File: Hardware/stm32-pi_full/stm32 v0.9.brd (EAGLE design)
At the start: 131.4 x 105.8 mm, 273 parts, among them J1 SOLDERJUMPERNO, Q1 MMBT3906, Q2 MMBT3904, Q3 MMBT3904, U1 ESP32-WROOM-32D, Y1 6MM_3.5MM_CRYSTAL

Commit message: minor, uipdate BoMs
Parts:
- R21: value 0R -> 2k
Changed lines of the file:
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@@
 <attribute name="VALUE" x="11.495" y="57.635" size="1.27" layer="27" rot="R270"/>
 </element>
-<element name="R21" library="resistor" package="R0603" value="0R" x="76.883209375" y="56.964225" smashed="yes">
+<element name="R21" library="resistor" package="R0603" value="2k" x="76.883209375" y="56.964225" smashed="yes">
 <attribute name="NAME" x="78.810725" y="59.036134375" size="1.27" layer="25" rot="R180"/>
 <attribute name="VALUE" x="76.248209375" y="55.059225" size="1.27" layer="27"/>

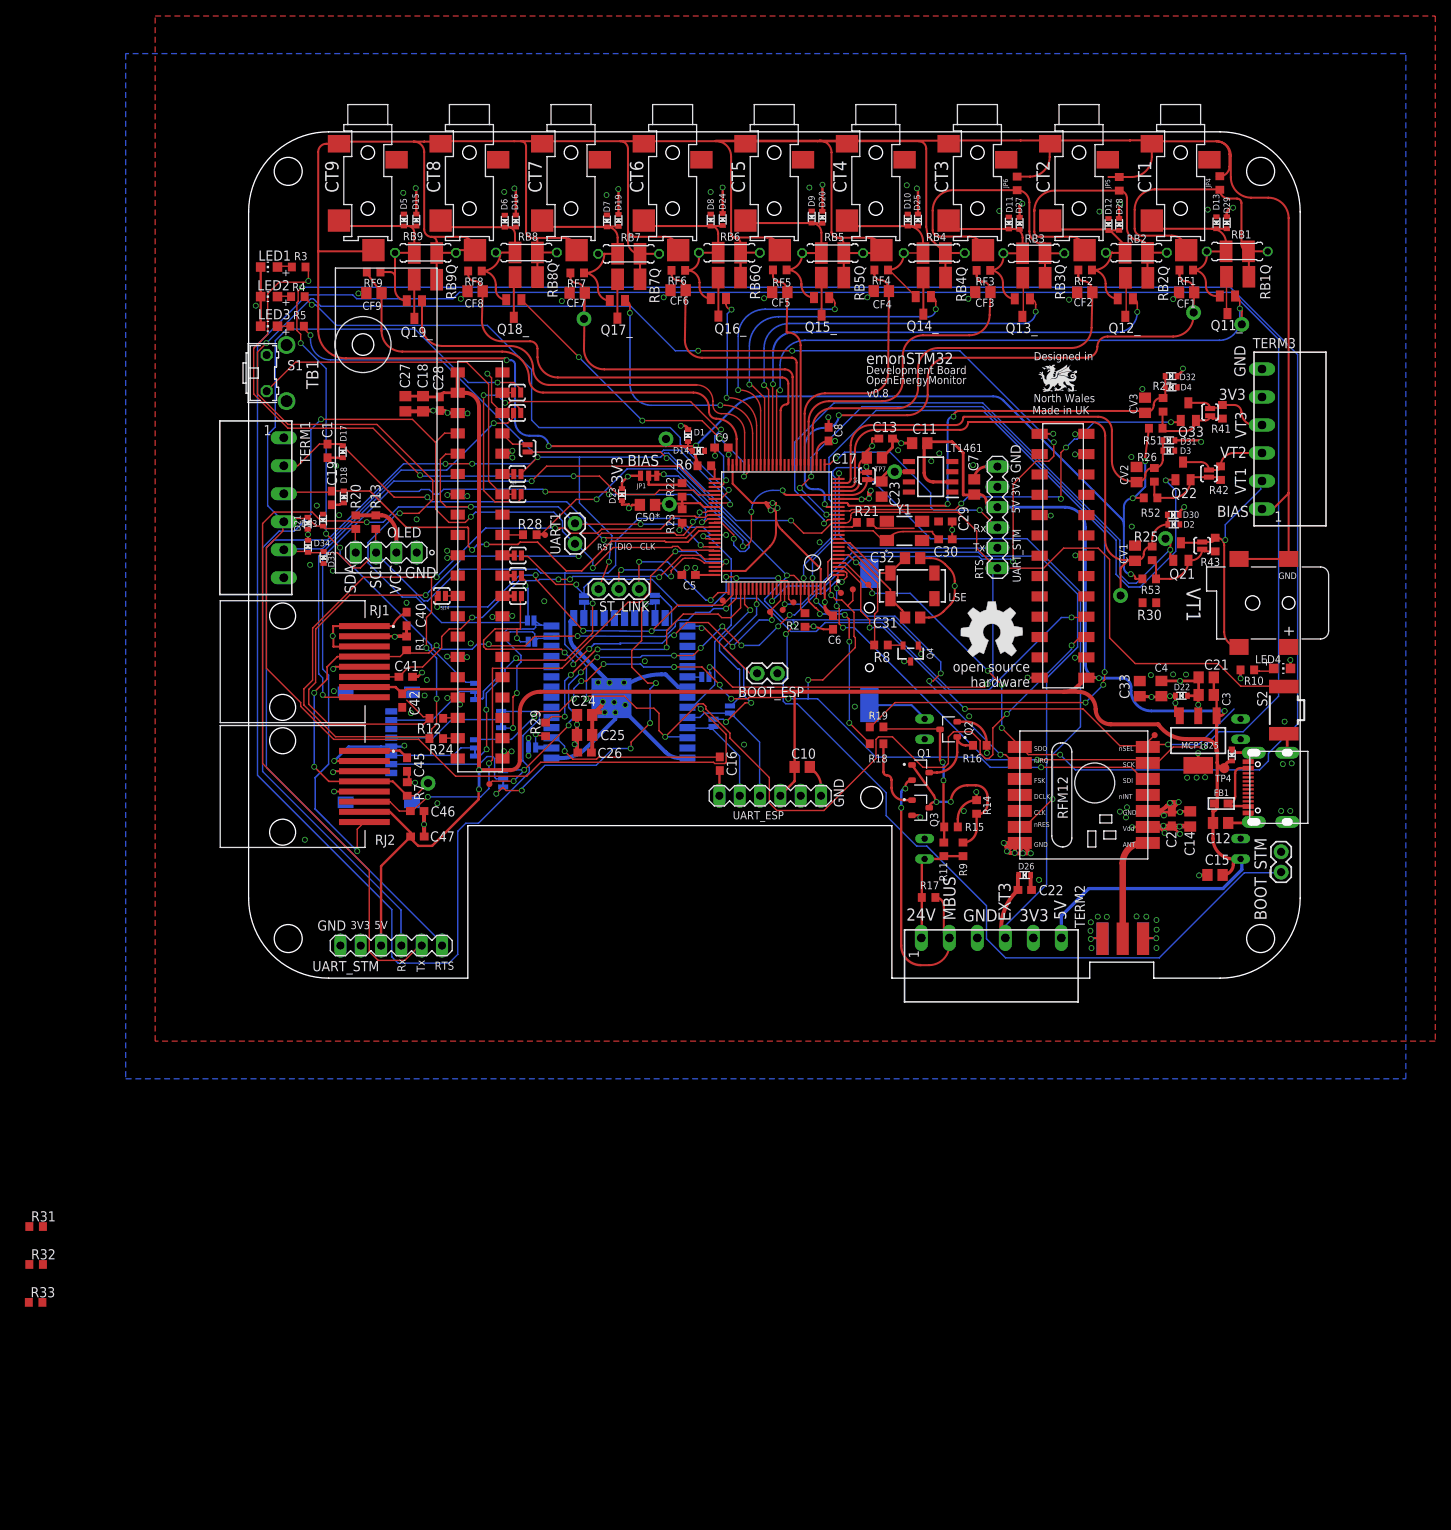
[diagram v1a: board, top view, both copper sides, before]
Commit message: minor changes, some checks on proto v0.8 done.
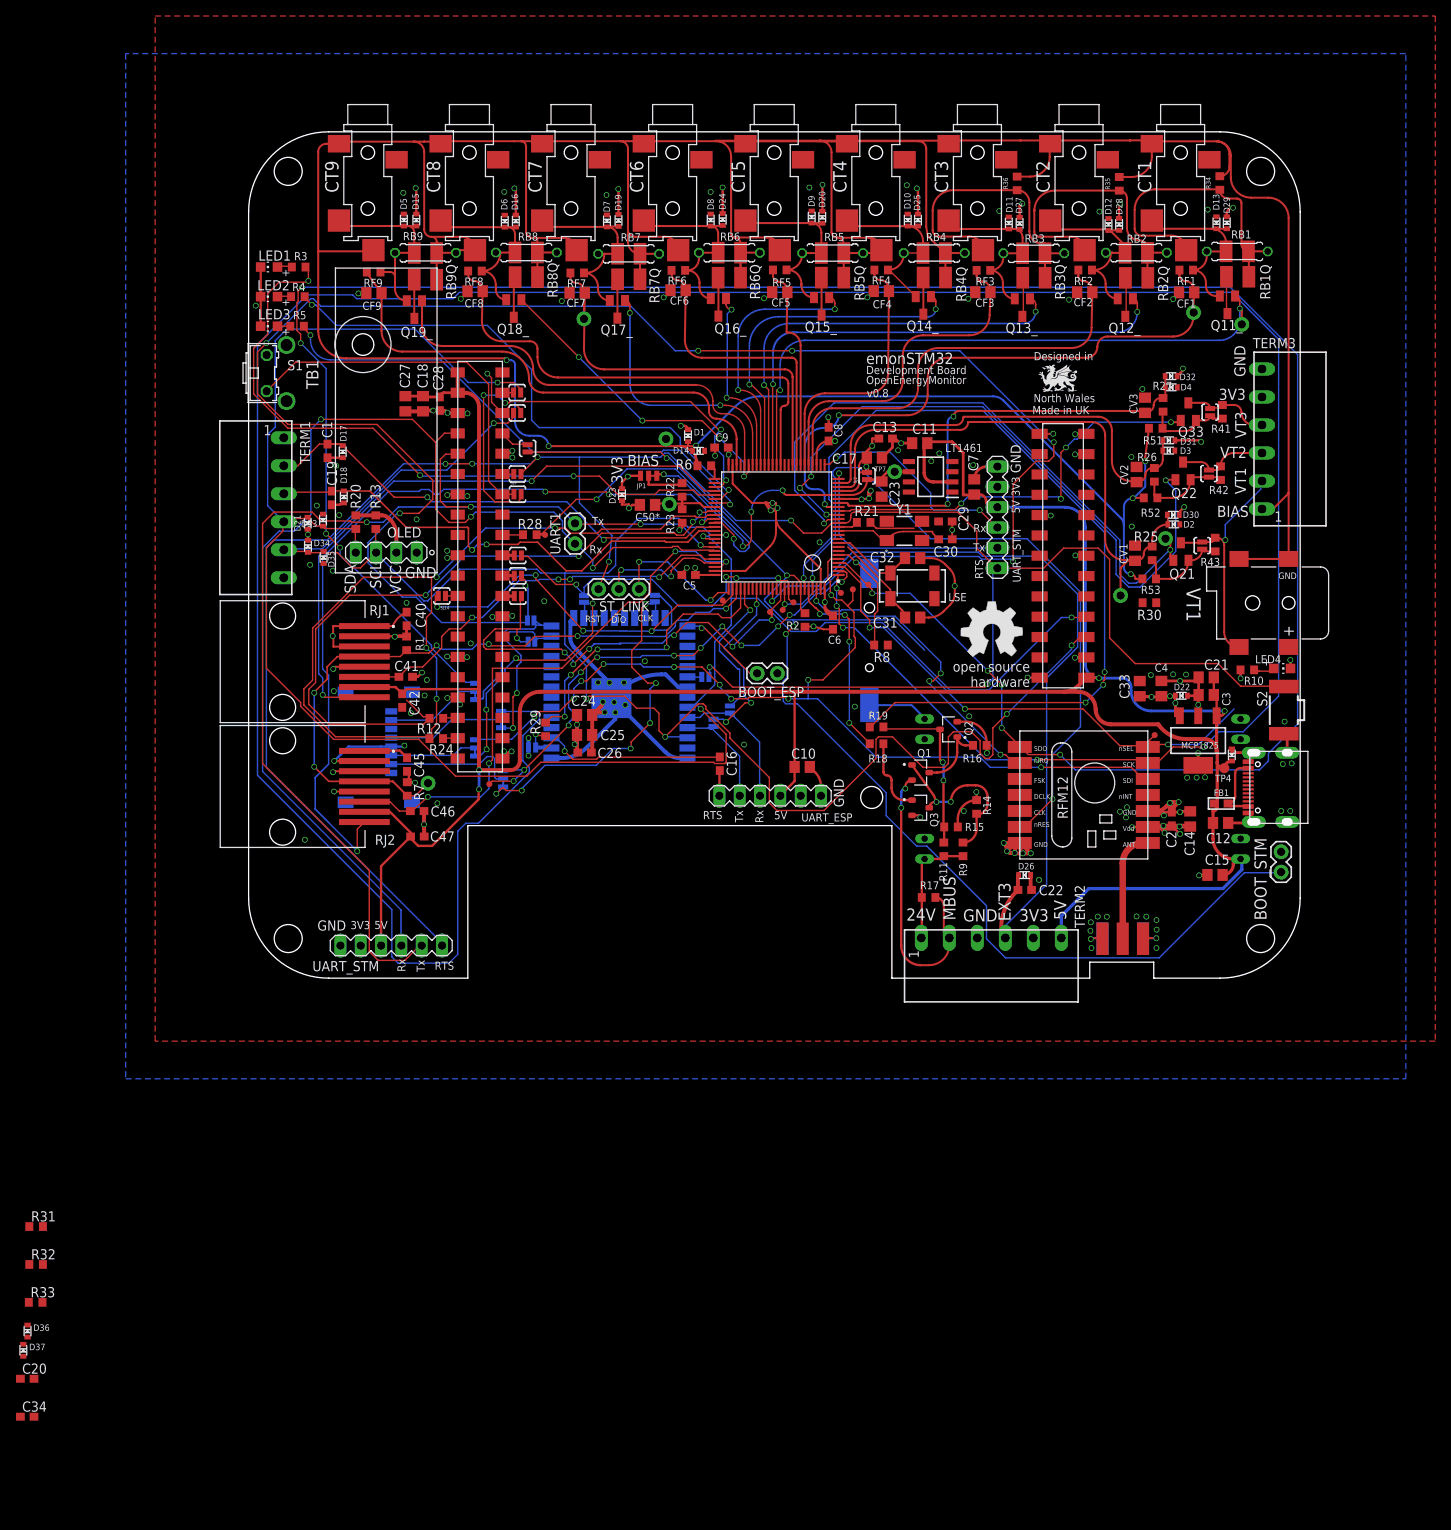
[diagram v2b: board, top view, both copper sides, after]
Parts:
- removed Q4: (no value), microbuilder:SOT23-R
- added C20, C34: 100nF, rcl:C0603
- added D36, D37: ESD5Z3.3T1G, microbuilder:SOD-523
- R34, R35, R36: value (none) -> 0R
- R8: value 1.5k -> 100k
- renumbered JP4 to R34, JP5 to R35, JP6 to R36
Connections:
- new net N$19: D37.K, R8.1
- net +3V3: no longer Q4.3
- net +5V: now also D36.A
- net GND: now also C20.2; no longer Q4.1
- net N$16: now also D36.K, D37.A; no longer Q4.2, R8.1
- net NRST_STM: now also C34.1, C34.2
- net VBAT: now also C20.1
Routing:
- net N$16: track 1.93 -> 0.00 mm
- net BIAS: track 588.4 -> 587.1 mm
- net GND: track 296.9 -> 295.6 mm, vias 143 -> 142
- net +3V3: track 143.8 -> 143.0 mm, vias 41 -> 40

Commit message: Various checks.
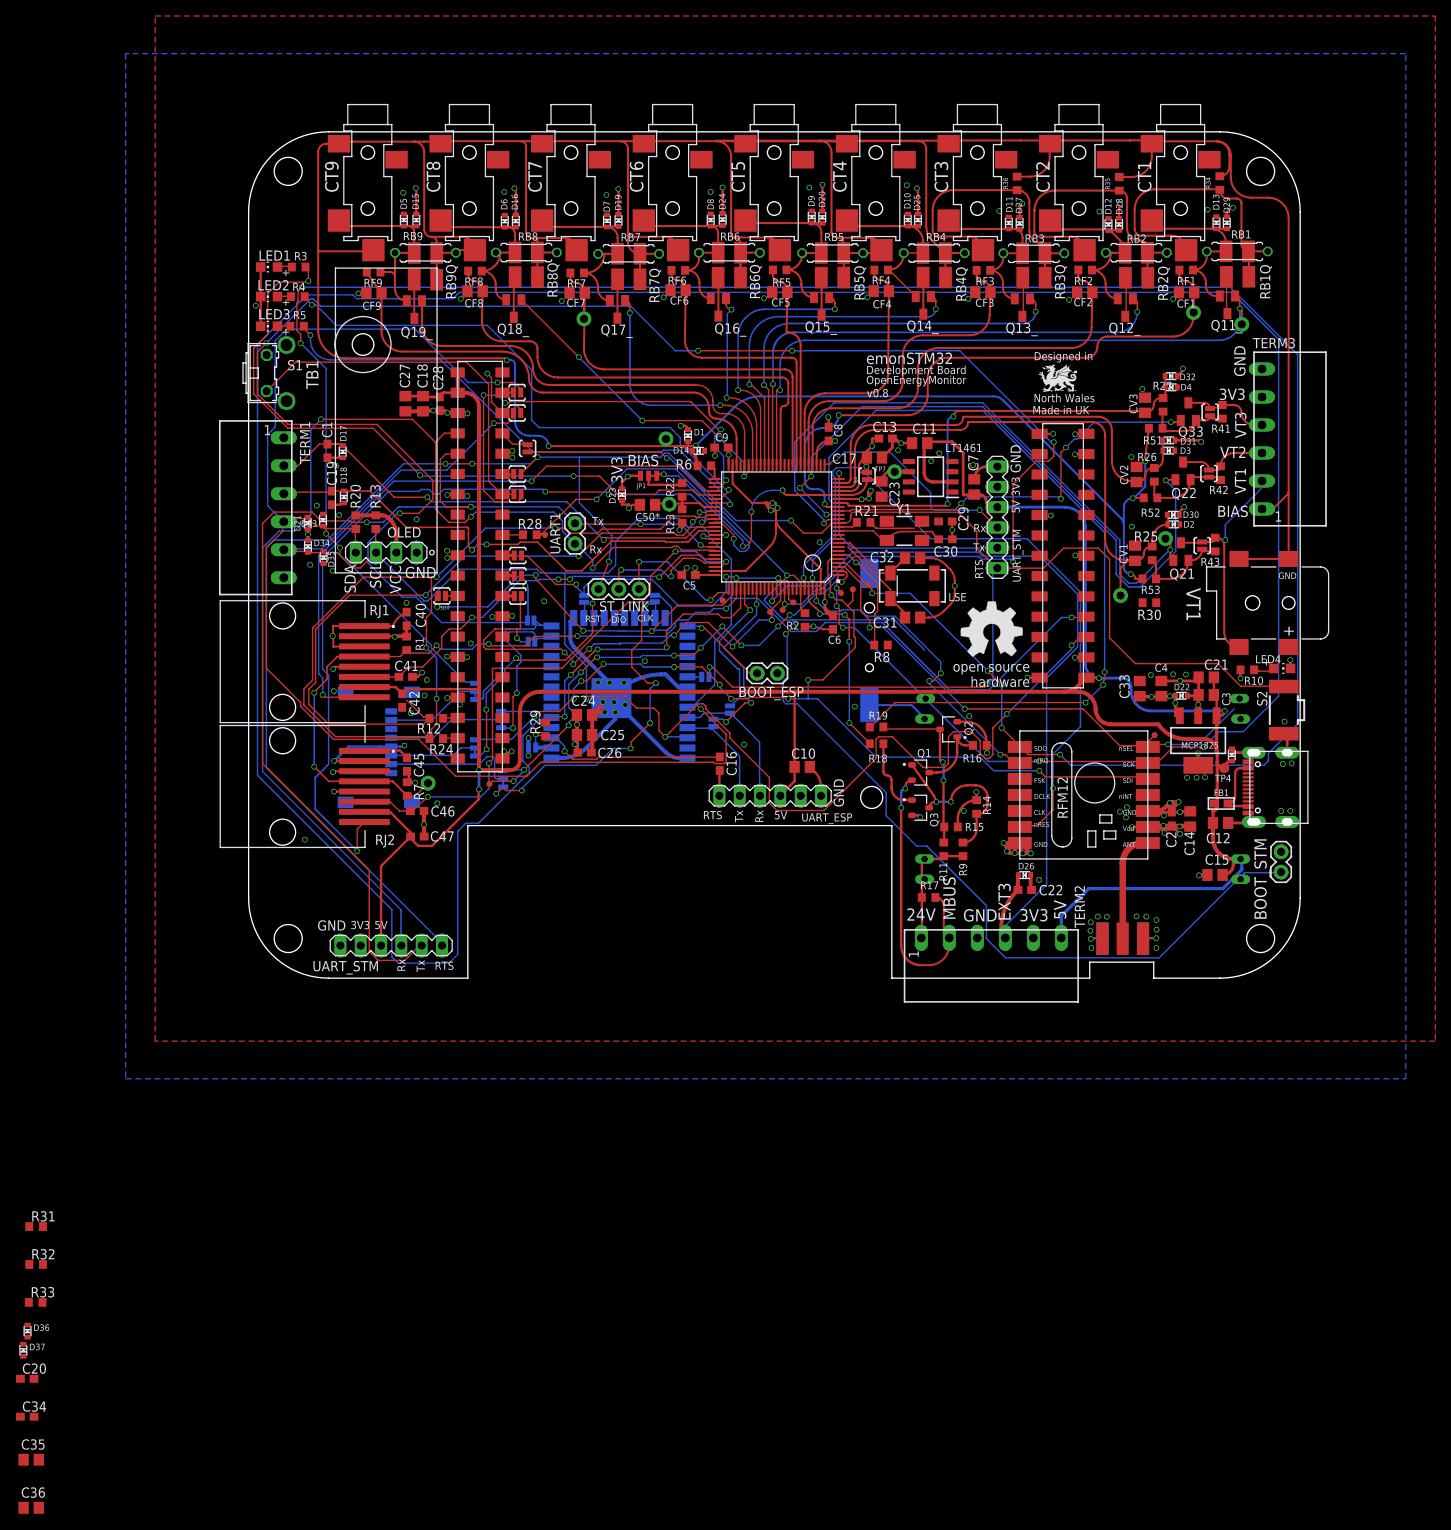
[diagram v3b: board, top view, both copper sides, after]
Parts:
- added C35, C36: 2.2uF, rcl:C0805
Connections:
- net BIAS: now also C35.1, C36.1
- net GND: now also C35.2, C36.2
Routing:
- net RST_RFM: track 86.5 -> 87.3 mm
